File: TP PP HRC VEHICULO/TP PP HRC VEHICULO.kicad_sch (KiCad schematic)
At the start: 56 parts, among them J10 Conn_01x04_Pin, J2 Conn_01x01_Pin, J3 Conn_01x01_Pin, J5vgnd1 Screw_Terminal_01x02, J6 Conn_01x04_Pin, J7 USB_B, J9 Conn_01x04_Pin, K1 Relay_SPDT, K2 Relay_SPDT, SW1 SW_Push, SW2 SW_Push, U1 ESP32-Devkit-V1, U2 LM317L_TO92

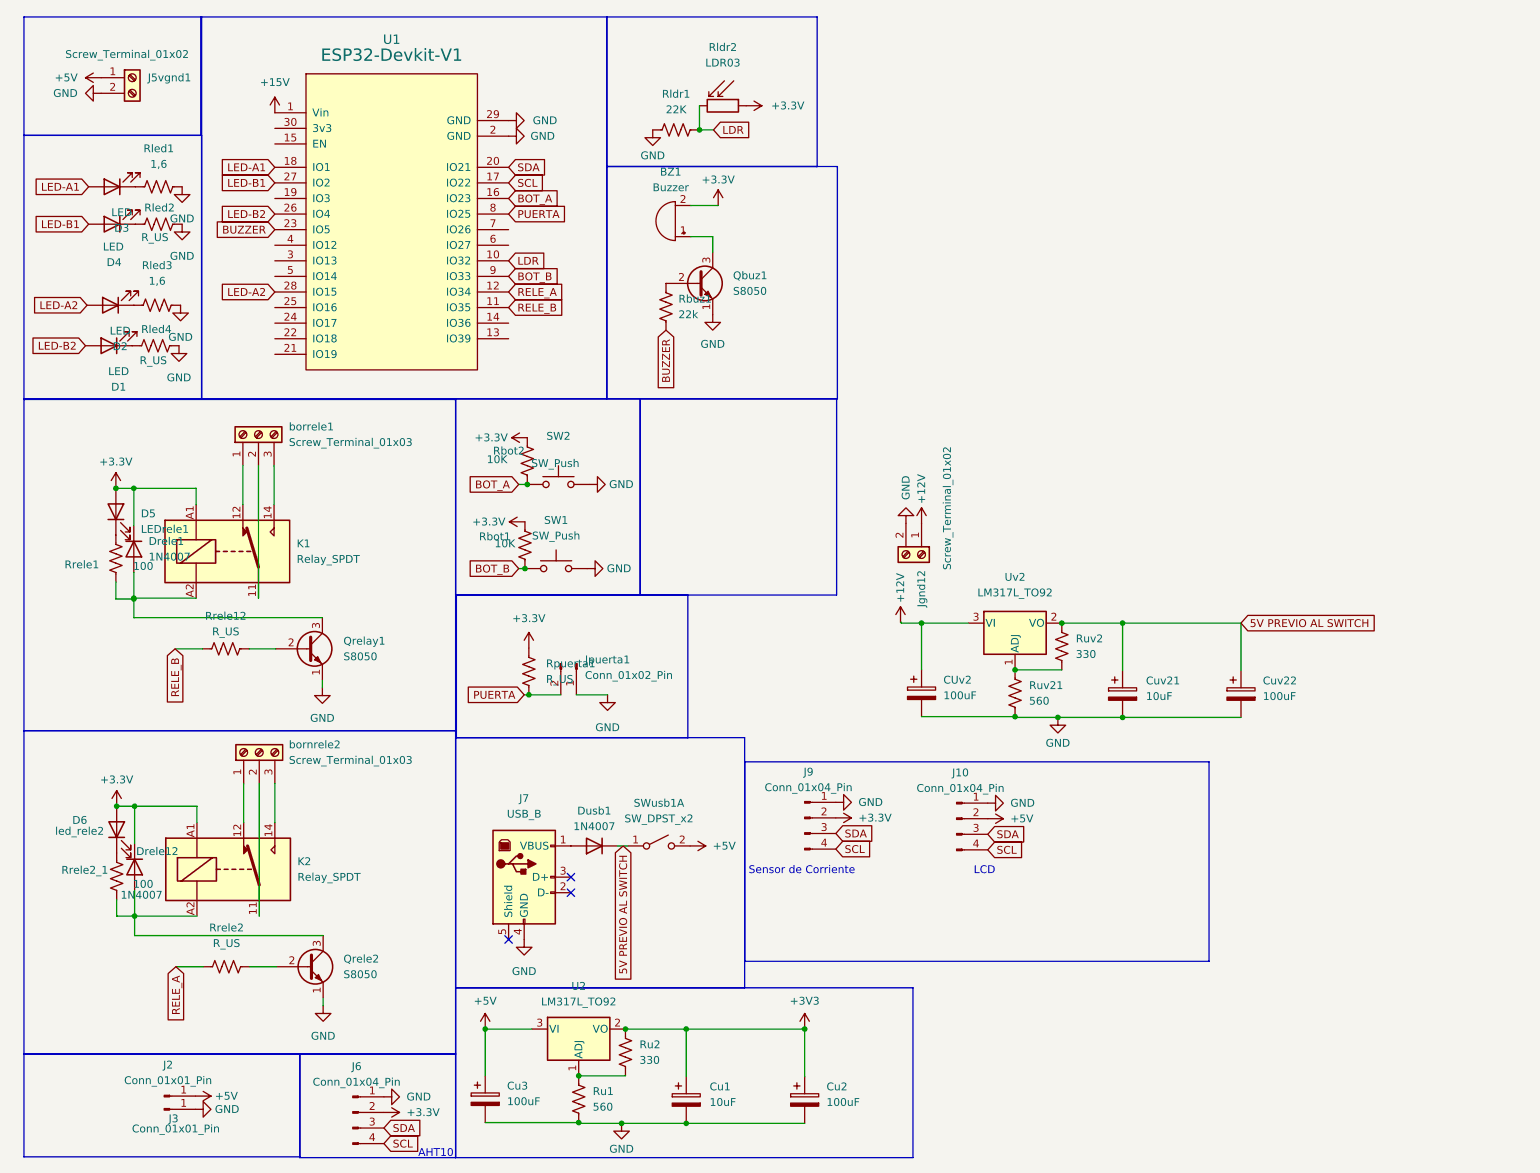
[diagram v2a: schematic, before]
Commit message: si
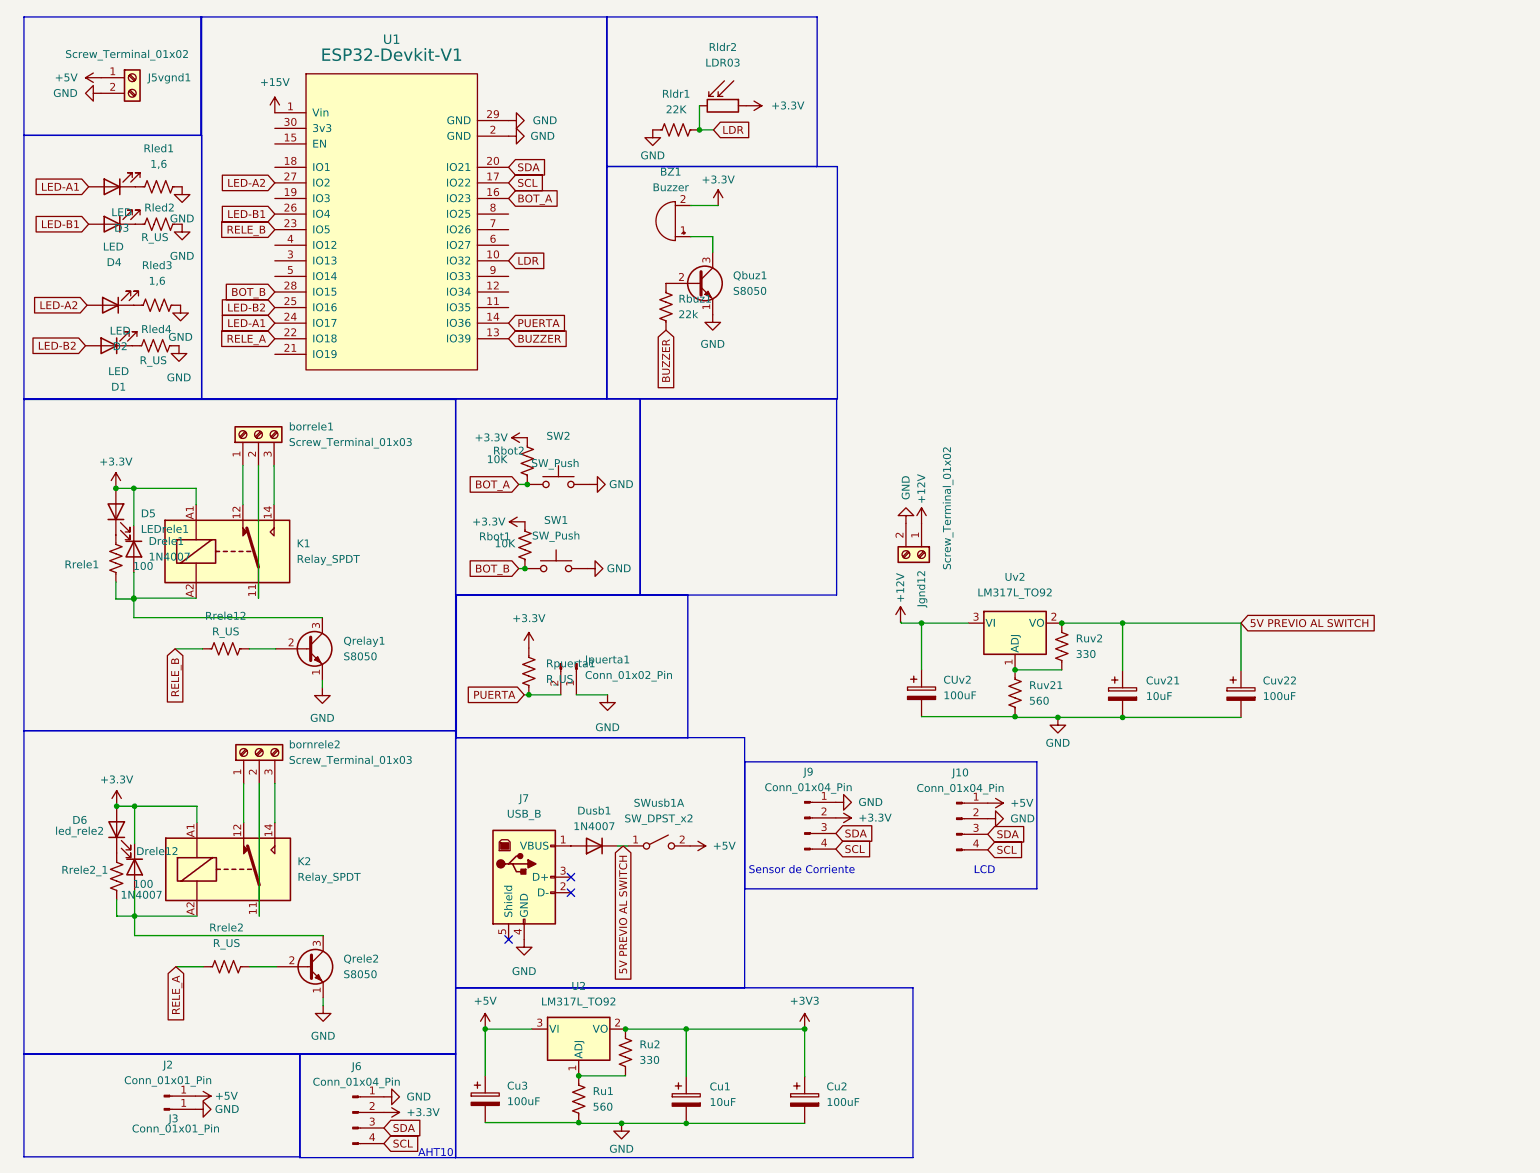
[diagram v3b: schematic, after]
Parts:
- D1, D2, D3, D4: footprint LED_THT:LED_D5.0mm -> Connector_Molex:Molex_KK-254_AE-6410-02A_1x02_P2.54mm_Vertical
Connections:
- net +5V: now also J10.1 (Pin_1); no longer J10.2 (Pin_2)
- net BOT_B: now also U1.28 (IO15); no longer U1.9 (IO33)
- net BUZZER: now also U1.13 (IO39); no longer U1.23 (IO5)
- net GND: now also J10.2 (Pin_2); no longer J10.1 (Pin_1)
- net LED-A1: now also U1.24 (IO17); no longer U1.18 (IO1)
- net LED-A2: now also U1.27 (IO2); no longer U1.28 (IO15)
- net LED-B1: now also U1.26 (IO4); no longer U1.27 (IO2)
- net LED-B2: now also U1.25 (IO16); no longer U1.26 (IO4)
- net PUERTA: now also U1.14 (IO36); no longer U1.8 (IO25)
- net RELE_A: now also U1.22 (IO18); no longer U1.12 (IO34)
- net RELE_B: now also U1.23 (IO5); no longer U1.11 (IO35)
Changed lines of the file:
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@@
 	(rectangle
 		(start 130.175 134.239)
-		(end 205.867 166.751)
+		(end 177.8 154.94)
 		(stroke
 			(width 0)
@@
 	(global_label "BOT_B"
 		(shape input)
-		(at 91.694 55.118 0)
+		(at 53.594 57.658 180)
 		(fields_autoplaced yes)
 		(effects
@@
 				(size 1.27 1.27)
 			)
-			(justify left)
+			(justify right)
 		)
 		(property "Intersheetrefs" "${INTERSHEET_REFS}"
-			(at 100.4849 55.118 0)
+			(at 44.8031 57.658 0)
 			(effects
 				(font
 					(size 1.27 1.27)
 				)
-				(justify left)
+				(justify right)
 				(hide yes)
 			)
@@
 	(global_label "BUZZER"
 		(shape input)
-		(at 53.594 47.498 180)
+		(at 91.694 65.278 0)
 		(fields_autoplaced yes)
 		(effects
@@
 				(size 1.27 1.27)
 			)
-			(justify right)
+			(justify left)
 		)
 		(property "Intersheetrefs" "${INTERSHEET_REFS}"
-			(at 43.1703 47.498 0)
+			(at 102.1177 65.278 0)
 			(effects
 				(font
 					(size 1.27 1.27)
 				)
-				(justify right)
+				(justify left)
 				(hide yes)
 			)
@@
 	(global_label "LED-A2"
 		(shape input)
-		(at 53.594 57.658 180)
+		(at 53.594 39.878 180)
 		(fields_autoplaced yes)
 		(effects
@@
 		)
 		(property "Intersheetrefs" "${INTERSHEET_REFS}"
-			(at 43.2912 57.658 0)
+			(at 43.2912 39.878 0)
 			(effects
 				(font
@@
 		)
 	)
-	(global_label "LED-B1"
-		(shape input)
-		(at 53.594 39.878 180)
-		(fields_autoplaced yes)
-		(effects
-			(font
-				(size 1.27 1.27)
-			)
-			(justify right)
-		)
-		(property "Intersheetrefs" "${INTERSHEET_REFS}"
-			(at 43.1098 39.878 0)
-			(effects
-				(font
-					(size 1.27 1.27)
-				)
-				(justify right)
-				(hide yes)
-			)
-		)
-	)
 	(global_label "SDA"
 		(shape input)
@@
 	(global_label "LED-B2"
 		(shape input)
-		(at 53.594 44.958 180)
+		(at 53.594 60.198 180)
 		(fields_autoplaced yes)
 		(effects
@@
 		)
 		(property "Intersheetrefs" "${INTERSHEET_REFS}"
-			(at 43.1098 44.958 0)
+			(at 43.1098 60.198 0)
 			(effects
 				(font
@@
 	(global_label "RELE_B"
 		(shape input)
-		(at 91.694 60.198 0)
+		(at 53.594 47.498 180)
 		(fields_autoplaced yes)
 		(effects
@@
 				(size 1.27 1.27)
 			)
-			(justify left)
+			(justify right)
 		)
 		(property "Intersheetrefs" "${INTERSHEET_REFS}"
-			(at 101.5129 60.198 0)
+			(at 43.7751 47.498 0)
 			(effects
 				(font
 					(size 1.27 1.27)
 				)
-				(justify left)
+				(justify right)
 				(hide yes)
 			)
@@
 		)
 	)
+	(global_label "LED-B1"
+		(shape input)
+		(at 53.594 44.958 180)
+		(fields_autoplaced yes)
+		(effects
+			(font
+				(size 1.27 1.27)
+			)
+			(justify right)
+		)
+		(property "Intersheetrefs" "${INTERSHEET_REFS}"
+			(at 43.1098 44.958 0)
+			(effects
+				(font
+					(size 1.27 1.27)
+				)
+				(justify right)
+				(hide yes)
+			)
+		)
+	)
 	(global_label "RELE_A"
 		(shape input)
-		(at 91.694 57.658 0)
+		(at 53.594 65.278 180)
 		(fields_autoplaced yes)
 		(effects
@@
 				(size 1.27 1.27)
 			)
-			(justify left)
+			(justify right)
 		)
 		(property "Intersheetrefs" "${INTERSHEET_REFS}"
-			(at 101.3315 57.658 0)
+			(at 43.9565 65.278 0)
 			(effects
 				(font
 					(size 1.27 1.27)
 				)
-				(justify left)
+				(justify right)
 				(hide yes)
 			)
@@
 	(global_label "LED-A1"
 		(shape input)
-		(at 53.594 37.338 180)
+		(at 53.594 62.738 180)
 		(fields_autoplaced yes)
 		(effects
@@
 		)
 		(property "Intersheetrefs" "${INTERSHEET_REFS}"
-			(at 43.2912 37.338 0)
+			(at 43.2912 62.738 0)
 			(effects
 				(font
@@
 	(global_label "PUERTA"
 		(shape input)
-		(at 91.694 44.958 0)
+		(at 91.694 62.738 0)
 		(fields_autoplaced yes)
 		(effects
@@
 		)
 		(property "Intersheetrefs" "${INTERSHEET_REFS}"
-			(at 101.7549 44.958 0)
+			(at 101.7549 62.738 0)
 			(effects
 				(font
@@
 	(symbol
 		(lib_id "power:GND")
-		(at 169.799 140.97 90)
+		(at 169.799 143.51 90)
 		(unit 1)
 		(exclude_from_sim no)
@@
 		(fields_autoplaced yes)
 		(property "Reference" "#PWR035"
-			(at 176.149 140.97 0)
+			(at 176.149 143.51 0)
 			(effects
 				(font
@@
 		)
 		(property "Value" "GND"
-			(at 173.482 140.97 90)
+			(at 173.482 143.51 90)
 			(effects
 				(font
@@
 		)
 		(property "Footprint" ""
-			(at 169.799 140.97 0)
+			(at 169.799 143.51 0)
 			(effects
 				(font
@@
 		)
 		(property "Datasheet" ""
-			(at 169.799 140.97 0)
+			(at 169.799 143.51 0)
 			(effects
 				(font
@@
 		)
 		(property "Description" ""
-			(at 169.799 140.97 0)
+			(at 169.799 143.51 0)
 			(effects
 				(font
@@
 	(symbol
 		(lib_id "power:+5V")
-		(at 169.799 143.51 270)
+		(at 169.799 140.97 270)
 		(unit 1)
 		(exclude_from_sim no)
@@
 		(fields_autoplaced yes)
 		(property "Reference" "#PWR036"
-			(at 165.989 143.51 0)
+			(at 165.989 140.97 0)
 			(effects
 				(font
@@
 		)
 		(property "Value" "+5V"
-			(at 173.482 143.51 90)
+			(at 173.482 140.97 90)
 			(effects
 				(font
@@
 		)
 		(property "Footprint" ""
-			(at 169.799 143.51 0)
+			(at 169.799 140.97 0)
 			(effects
 				(font
@@
 		)
 		(property "Datasheet" ""
-			(at 169.799 143.51 0)
+			(at 169.799 140.97 0)
 			(effects
 				(font
@@
 		)
 		(property "Description" ""
-			(at 169.799 143.51 0)
+			(at 169.799 140.97 0)
 			(effects
 				(font
@@
 			)
 		)
-		(property "Footprint" "LED_THT:LED_D5.0mm"
+		(property "Footprint" "Connector_Molex:Molex_KK-254_AE-6410-02A_1x02_P2.54mm_Vertical"
 			(at 26.797 59.817 0)
 			(effects
@@
 			)
 		)
-		(property "Footprint" "LED_THT:LED_D5.0mm"
+		(property "Footprint" "Connector_Molex:Molex_KK-254_AE-6410-02A_1x02_P2.54mm_Vertical"
 			(at 27.051 46.609 0)
 			(effects
@@
 			)
 		)
-		(property "Footprint" "LED_THT:LED_D5.0mm"
+		(property "Footprint" "Connector_Molex:Molex_KK-254_AE-6410-02A_1x02_P2.54mm_Vertical"
 			(at 27.051 40.513 0)
 			(effects
@@
 			)
 		)
-		(property "Footprint" "LED_THT:LED_D5.0mm"
+		(property "Footprint" "Connector_Molex:Molex_KK-254_AE-6410-02A_1x02_P2.54mm_Vertical"
 			(at 26.543 66.421 0)
 			(effects

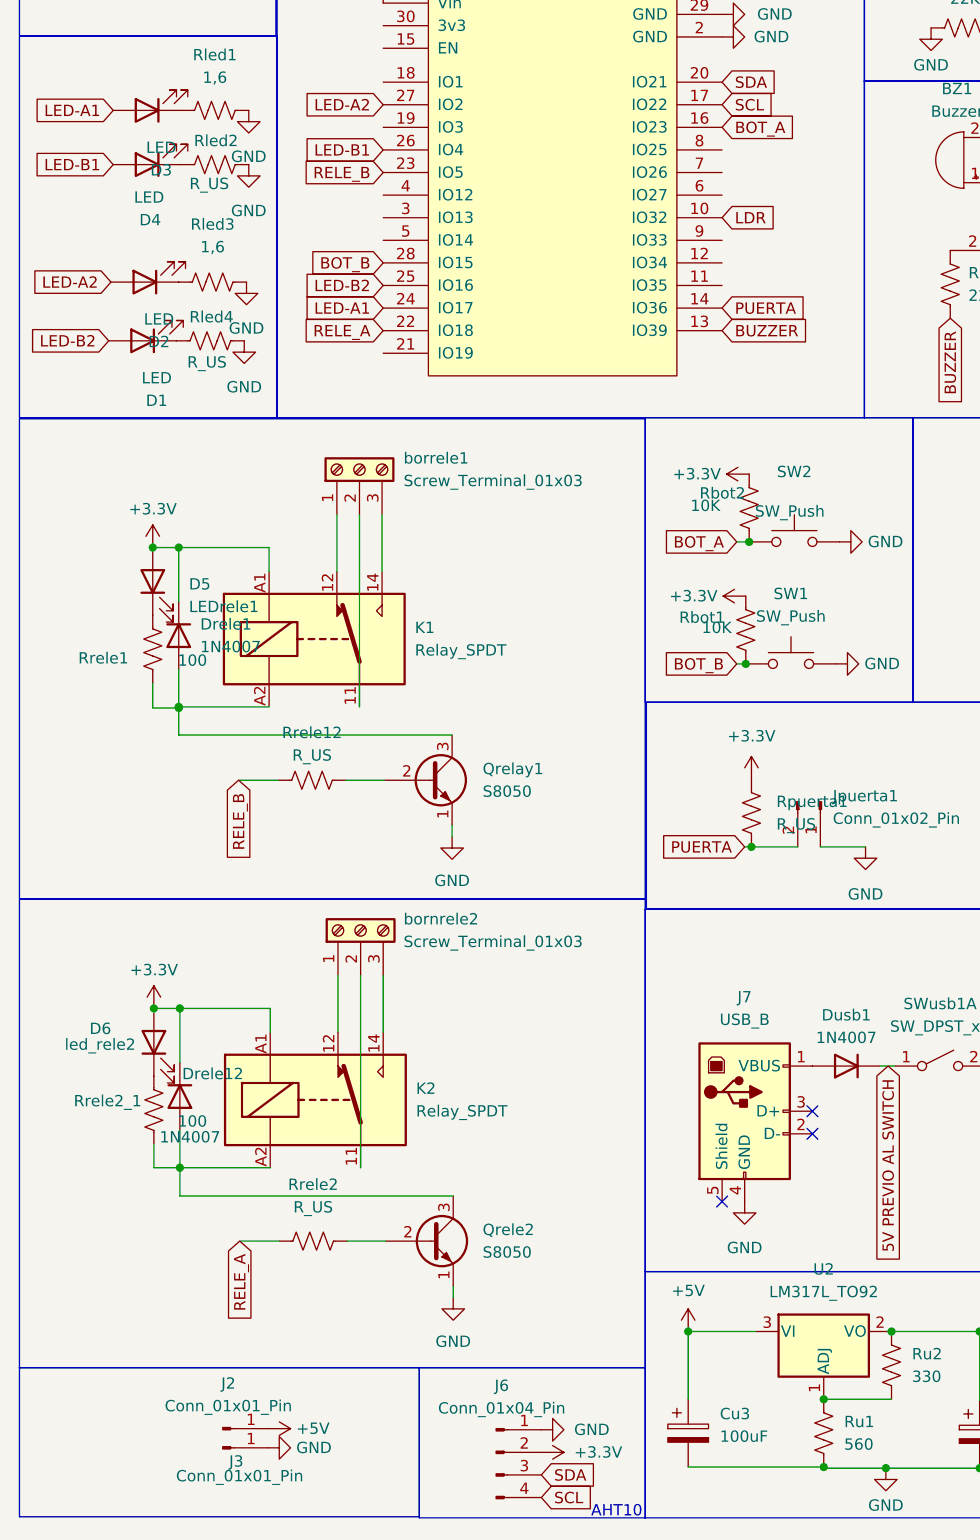
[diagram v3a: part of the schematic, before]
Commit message: aa
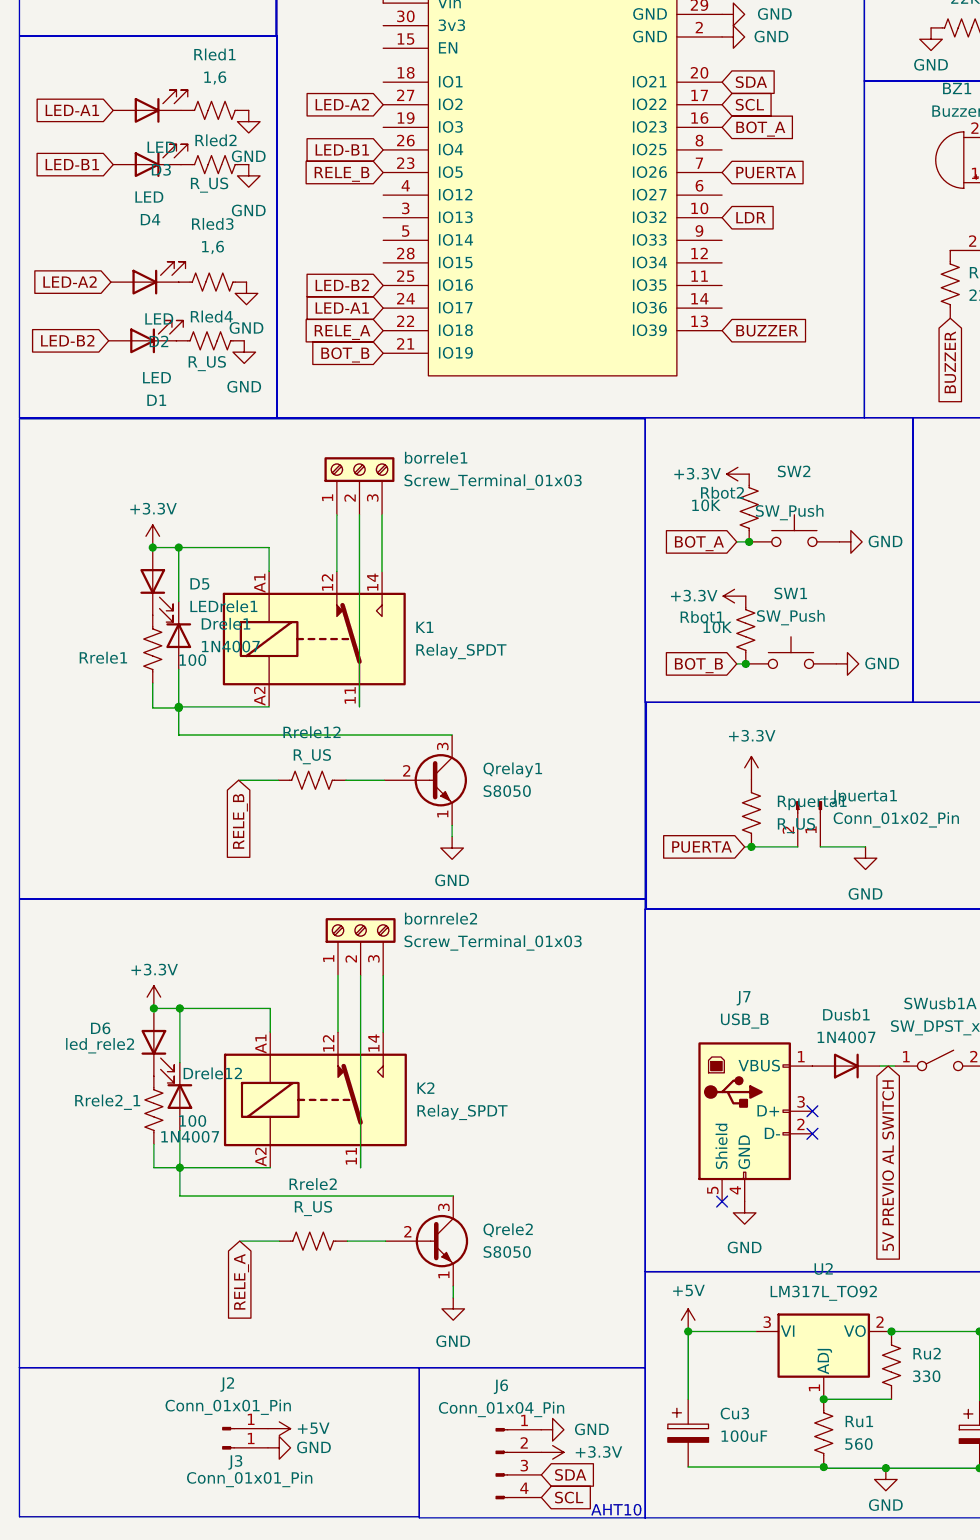
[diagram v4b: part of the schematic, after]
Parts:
- J2, J3: footprint Connector_Molex:Molex_KK-254_AE-6410-04A_1x04_P2.54mm_Vertical -> Connector_PinHeader_2.54mm:PinHeader_1x01_P2.54mm_Vertical
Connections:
- net BOT_B: now also U1.21 (IO19); no longer U1.28 (IO15)
- net PUERTA: now also U1.7 (IO26); no longer U1.14 (IO36)
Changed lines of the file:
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@@
 		)
 	)
-	(global_label "BOT_B"
-		(shape input)
-		(at 53.594 57.658 180)
-		(fields_autoplaced yes)
-		(effects
-			(font
-				(size 1.27 1.27)
-			)
-			(justify right)
-		)
-		(property "Intersheetrefs" "${INTERSHEET_REFS}"
-			(at 44.8031 57.658 0)
-			(effects
-				(font
-					(size 1.27 1.27)
-				)
-				(justify right)
-				(hide yes)
-			)
-		)
-	)
 	(global_label "BUZZER"
 		(shape input)
@@
 		)
 	)
+	(global_label "BOT_B"
+		(shape input)
+		(at 53.594 67.818 180)
+		(fields_autoplaced yes)
+		(effects
+			(font
+				(size 1.27 1.27)
+			)
+			(justify right)
+		)
+		(property "Intersheetrefs" "${INTERSHEET_REFS}"
+			(at 44.8031 67.818 0)
+			(effects
+				(font
+					(size 1.27 1.27)
+				)
+				(justify right)
+				(hide yes)
+			)
+		)
+	)
 	(global_label "LED-B1"
 		(shape input)
@@
 	(global_label "PUERTA"
 		(shape input)
-		(at 91.694 62.738 0)
+		(at 91.694 47.498 0)
 		(fields_autoplaced yes)
 		(effects
@@
 		)
 		(property "Intersheetrefs" "${INTERSHEET_REFS}"
-			(at 101.7549 62.738 0)
+			(at 101.7549 47.498 0)
 			(effects
 				(font
@@
 		)
 		(property "Value" "Conn_01x01_Pin"
-			(at 37.465 194.056 0)
+			(at 38.608 194.31 0)
 			(effects
 				(font
@@
 			)
 		)
-		(property "Footprint" "Connector_Molex:Molex_KK-254_AE-6410-04A_1x04_P2.54mm_Vertical"
+		(property "Footprint" "Connector_PinHeader_2.54mm:PinHeader_1x01_P2.54mm_Vertical"
 			(at 35.56 190.881 0)
 			(effects
@@
 			)
 		)
-		(property "Footprint" "Connector_Molex:Molex_KK-254_AE-6410-04A_1x04_P2.54mm_Vertical"
+		(property "Footprint" "Connector_PinHeader_2.54mm:PinHeader_1x01_P2.54mm_Vertical"
 			(at 35.56 188.722 0)
 			(effects
